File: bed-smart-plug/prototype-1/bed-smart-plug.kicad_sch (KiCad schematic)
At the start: 24 parts, among them J1 Main, J2 Prises, J3 Triac gate protection, J4 Triac snubber, J5 Opto snubber, J6 Opto snubber 2, Q1 BT136-600, U1 MOC3021M, U5 ESP32-POE-ISO, U6 RXB6

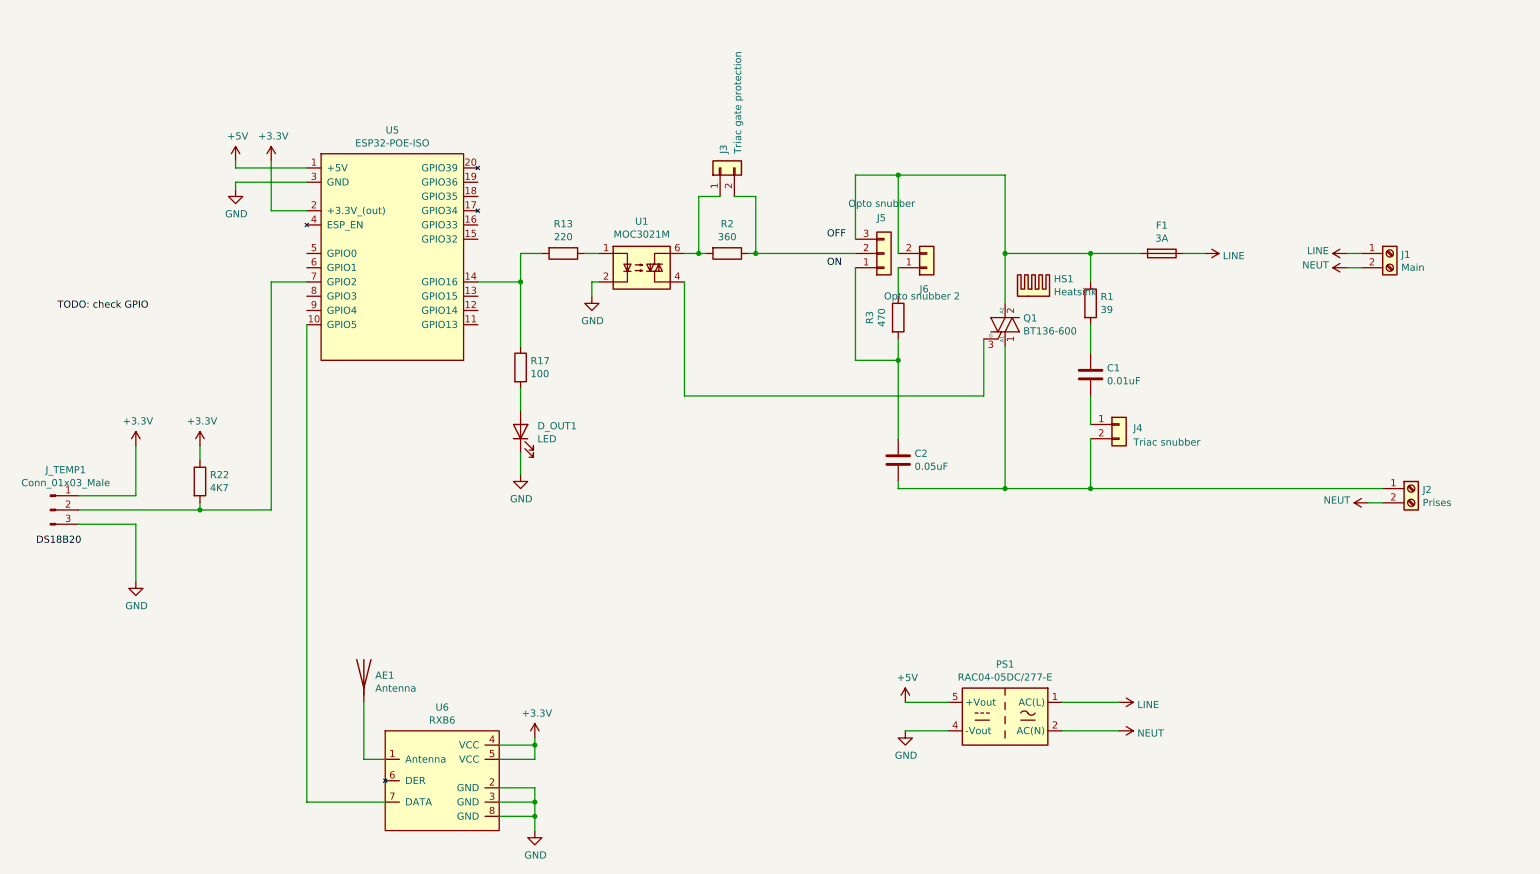
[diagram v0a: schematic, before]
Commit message: wip schematics
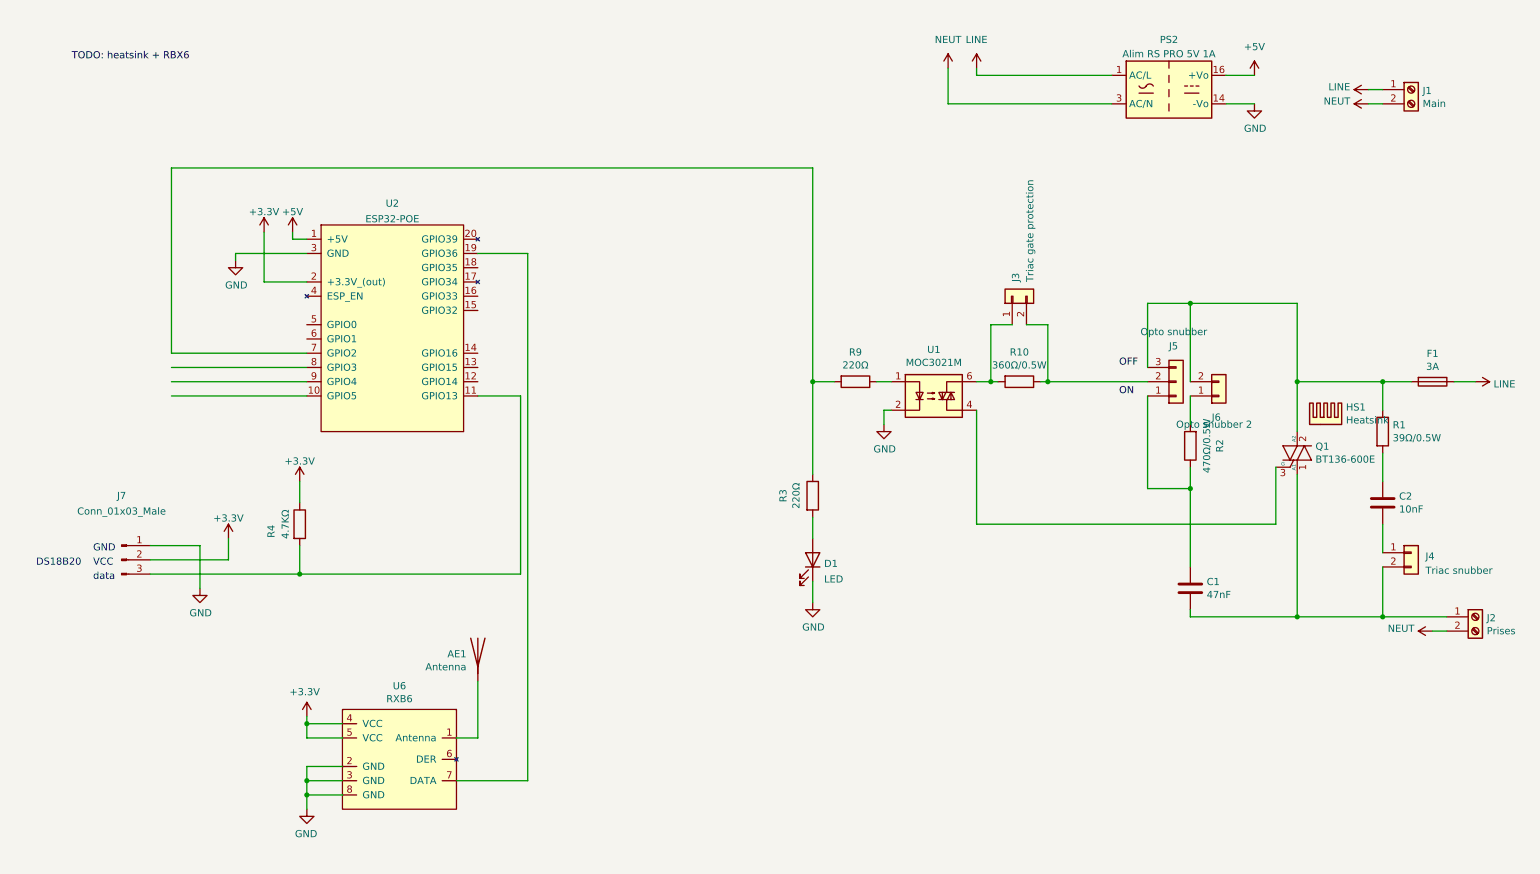
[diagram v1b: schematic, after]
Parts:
- removed D_OUT1: LED, LED_SMD:LED_1206_3216Metric_Pad1.42x1.75mm_HandSolder, symbol Device:LED
- removed J_TEMP1: Conn_01x03_Male, Connector_PinHeader_2.54mm:PinHeader_1x03_P2.54mm_Vertical, symbol Connector:Conn_01x03_Male
- removed PS1: RAC04-05DC/277-E, Converter_ACDC:Converter_ACDC_RECOM_RAC04-xxSGx_THT, symbol Converter_ACDC:RAC04-05SGA
- removed R13: 220, Resistor_SMD:R_1206_3216Metric_Pad1.42x1.75mm_HandSolder, symbol Device:R
- removed R17: 100, Resistor_SMD:R_1206_3216Metric_Pad1.42x1.75mm_HandSolder, symbol Device:R
- removed R22: 4K7, Resistor_SMD:R_1206_3216Metric_Pad1.42x1.75mm_HandSolder, symbol Device:R
- removed U5: ESP32-POE-ISO, symbol mylife-symbols:ESP32-POE-ISO
- added D1: LED, Diode_SMD:D_0805_2012Metric, symbol Device:LED
- added J7: Conn_01x03_Male, Connector_PinHeader_2.54mm:PinHeader_1x03_P2.54mm_Vertical, symbol Connector:Conn_01x03_Male
- added PS2: Alim RS PRO 5V 1A, Converter_ACDC:Converter_ACDC_MeanWell_IRM-03-xx_THT, symbol Converter_ACDC:IRM-03-5
- added R10: 360Ω/0.5W, Resistor_SMD:R_1210_3225Metric, symbol Device:R
- added R4: 4.7KΩ, Resistor_SMD:R_0402_1005Metric, symbol Device:R
- added R9: 220Ω, Resistor_SMD:R_0603_1608Metric, symbol Device:R
- added U2: ESP32-POE, mylife-footprints:ESP32-POE, symbol mylife-symbols:ESP32-POE-ISO
- C1: value 0.01uF -> 47nF; footprint Capacitor_THT:C_Rect_L9.0mm_W2.5mm_P7.50mm_MKT -> Capacitor_SMD:C_1206_3216Metric; LCSC (none) -> C309031
- C2: value 0.05uF -> 10nF; footprint Capacitor_SMD:C_2220_5650Metric_Pad1.97x5.40mm_HandSolder -> Capacitor_SMD:C_0805_2012Metric; LCSC (none) -> C106840
- J3, J4, J6: footprint (none) -> Connector_PinHeader_2.54mm:PinHeader_1x02_P2.54mm_Vertical
- J5: footprint (none) -> Connector_PinHeader_2.54mm:PinHeader_1x03_P2.54mm_Vertical
- Q1: value BT136-600 -> BT136-600E
- R1: value 39 -> 39Ω/0.5W; footprint Resistor_THT:R_Axial_DIN0204_L3.6mm_D1.6mm_P7.62mm_Horizontal -> Resistor_SMD:R_1210_3225Metric; LCSC (none) -> C422307
- R2: value 360 -> 470Ω/0.5W; footprint Resistor_SMD:R_1206_3216Metric_Pad1.42x1.75mm_HandSolder -> Resistor_SMD:R_1210_3225Metric; LCSC (none) -> C830186
- R3: value 470 -> 220Ω; footprint Resistor_SMD:R_1206_3216Metric_Pad1.42x1.75mm_HandSolder -> Resistor_SMD:R_0603_1608Metric; LCSC (none) -> C22962
- U1: footprint Package_DIP:DIP-6_W8.89mm_SMDSocket_LongPads -> Package_DIP:SMDIP-6_W9.53mm; LCSC (none) -> C108500
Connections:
- net +3V3: now also J7.2 (Pin_2), R4.1, U2.2 (+3.3V_(out))
- net +5V: now also PS2.16 (+Vo), U2.1 (+5V)
- net GND: now also D1.1 (K), J7.1 (Pin_1), PS2.14 (-Vo), U2.3 (GND)
- net LINE: now also PS2.1 (AC/L)
- net NEUT: now also PS2.3 (AC/N)
- net at U1.1: now also R9.1
- net at J3.1 (Pin_1), U1.6: now also R10.2; no longer R2.2
- net at J2.1 (Pin_1), J4.2 (Pin_2), Q1.1 (A1): now also C1.2; no longer C2.2
- net at R1.2: now also C2.1; no longer C1.1
- net at J3.2 (Pin_2), J5.2 (Pin_2): now also R10.1; no longer R2.1
- net at R3.1: now also R9.2, U2.7 (GPIO2); no longer J6.1 (Pin_1)
- net at J4.1 (Pin_1): now also C2.2; no longer C1.2
- net at U6.7 (DATA): now also U2.19 (GPIO36)
- new net: J7.3 (Pin_3), R4.2, U2.11 (GPIO13)
- new net: D1.2 (A), R3.2
- new net: C1.1, J5.1 (Pin_1), R2.1
- new net: J6.1 (Pin_1), R2.2
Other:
- note added: "DS18B20"
- note added: "GND"
- note added: "VCC"
- note added: "data"
- moved on the sheet: AE1, F1, HS1, J1, J2, J3, J4, J5, J6, Q1, U1, U6
